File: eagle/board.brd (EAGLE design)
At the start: 53 x 50 mm, 31 parts

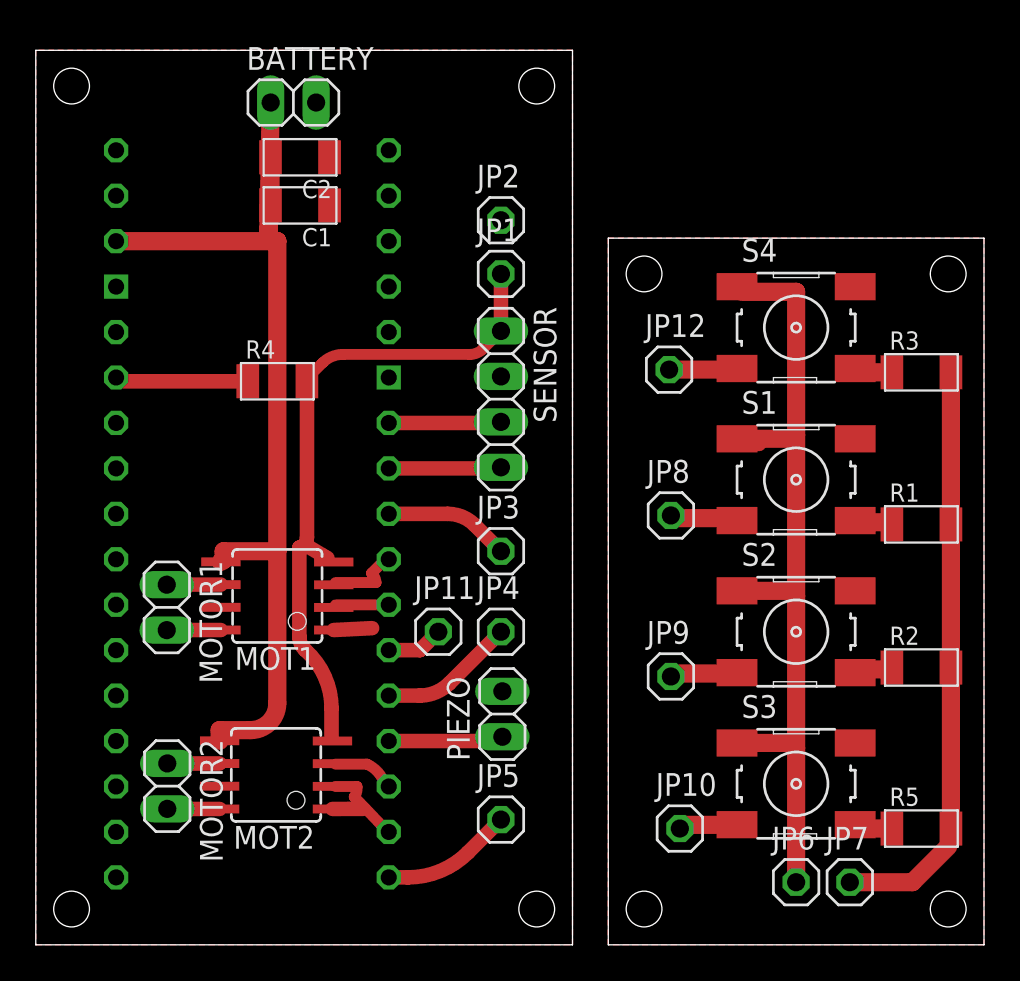
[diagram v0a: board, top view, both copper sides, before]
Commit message: pcb update
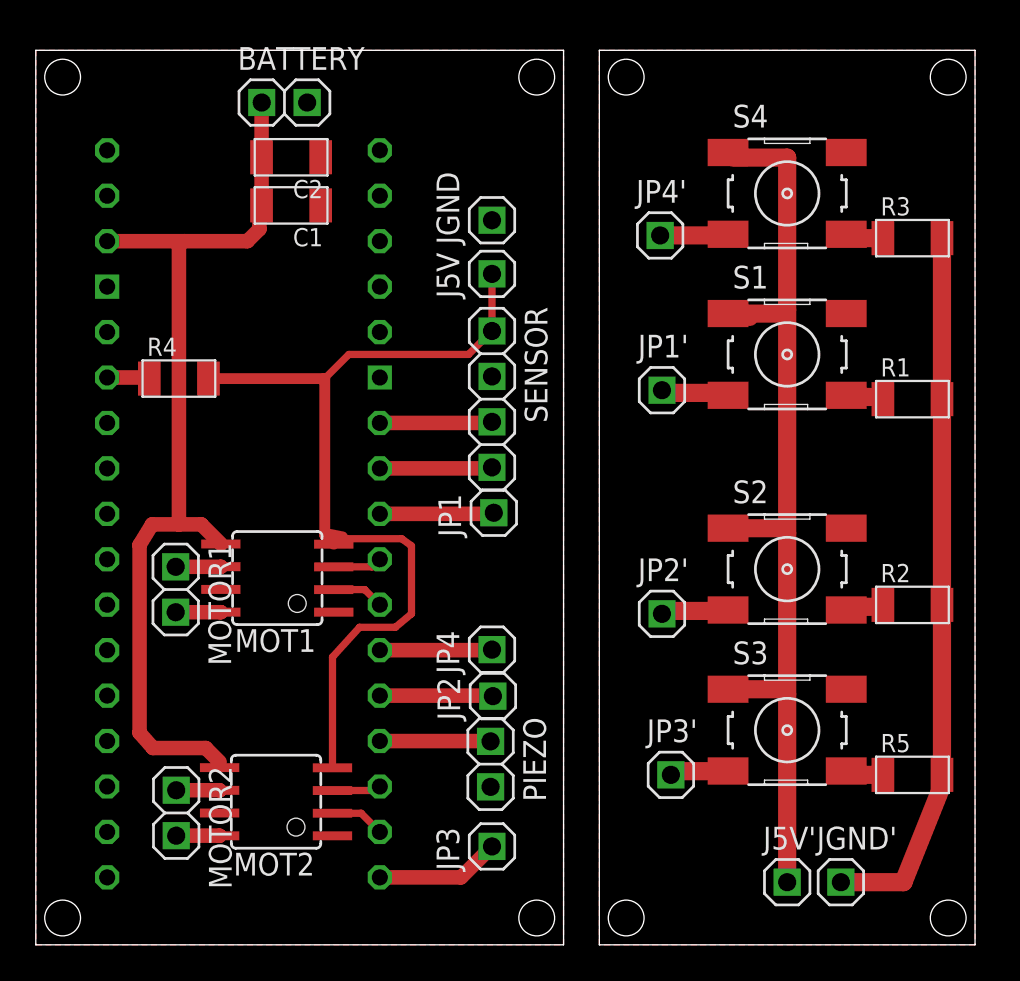
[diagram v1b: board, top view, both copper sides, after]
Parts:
- removed JP10, JP11, JP12, JP5, JP6, JP7, JP8, JP9: (no value), pinhead:1X01
- added J5V, J5V', JGND, JGND', JP1', JP2', JP3', JP4': (no value), pinhead:1X01
- moved JP2 26.6 mm to (25.6, 13.9), turned to 90 degrees
- moved JP3 16.5 mm to (25.5, 5.50), turned to 90 degrees
- moved JP1 13.4 mm to (25.6, 24.1), turned to 90 degrees
- moved R3 7.52 mm to (49.0, 39.5)
- moved S4 7.52 mm to (42.0, 42.0)
- moved R1 7.02 mm to (49.0, 30.5)
- moved S1 7.02 mm to (42.0, 33.0)
- moved R4 5.50 mm to (8.00, 31.6)
- moved R2 3.54 mm to (49.0, 19.0)
- moved S2 3.54 mm to (42.0, 21.0)
- moved R5 3.04 mm to (49.0, 9.50)
- moved S3 3.04 mm to (42.0, 12.0)
- moved PIEZO 2.88 mm to (25.4, 10.1), turned to 270 degrees
- moved MOTOR2 1.58 mm to (7.85, 7.37)
- moved MOT2 1.50 mm to (13.4, 8.00)
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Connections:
- net 5V: now also J5V.1; no longer JP1.1
- net 5V': now also J5V'.1; no longer JP6.1
- net BUT1: now also JP1.1; no longer JP3.1
- net BUT1': now also JP1'.1; no longer JP8.1
- net BUT2: now also JP2.1; no longer JP4.1
- net BUT2': now also JP2'.1; no longer JP9.1
- net BUT3: now also JP3.1; no longer JP5.1
- net BUT3': now also JP3'.1; no longer JP10.1
- net BUT4: now also JP4.1; no longer JP11.1
- net BUT4': now also JP4'.1; no longer JP12.1
- net GND: now also JGND.1; no longer JP2.1
- net GND': now also JGND'.1; no longer JP7.1
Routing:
- net 5V: track 37.7 -> 50.0 mm
- net 5V': track 48.0 -> 55.5 mm
- net GND': track 33.2 -> 40.3 mm
- net N$3: track 7.56 -> 2.38 mm
- net GND: track 3.86 -> 0.00 mm
- net BUT4: track 3.19 -> 6.28 mm
- net MOT2-2: track 4.72 -> 3.08 mm
- net VIN: track 55.1 -> 53.5 mm
- net MOT1-1: track 4.27 -> 2.75 mm
- net BUT2: track 7.60 -> 6.33 mm
- net MOT2-1: track 3.68 -> 2.74 mm
- net BUT1: track 7.00 -> 6.39 mm
- net MOT1-OUT2: track 3.03 -> 2.53 mm
- net MOT1-OUT1: track 3.03 -> 2.53 mm
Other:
- board size 53 x 50 mm -> 52.5 x 50 mm
